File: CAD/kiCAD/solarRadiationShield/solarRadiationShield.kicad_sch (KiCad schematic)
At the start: 4 parts, among them J3 INSIG

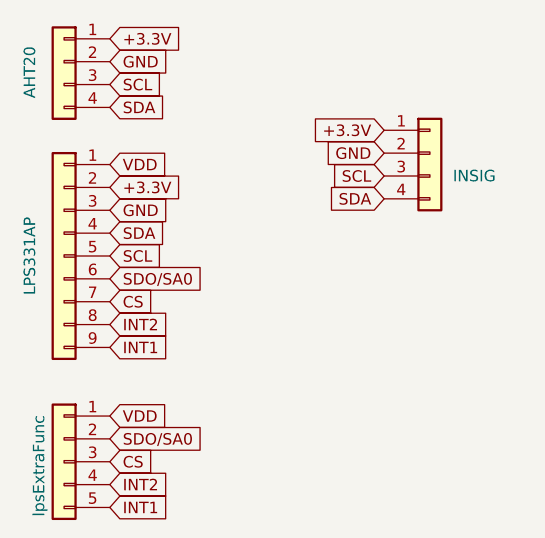
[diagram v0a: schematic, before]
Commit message: Big Updates
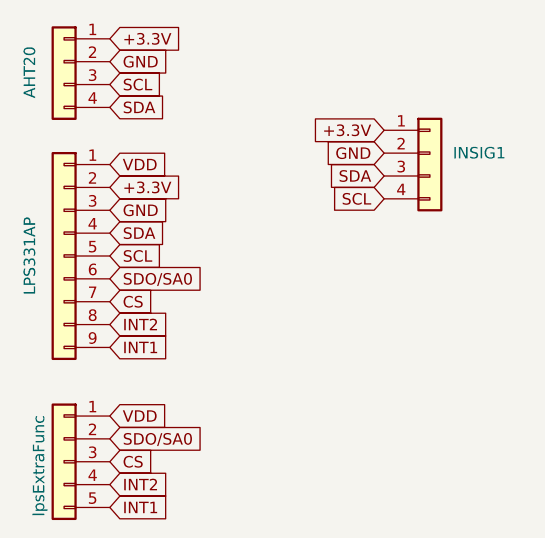
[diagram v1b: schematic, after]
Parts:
- renumbered J3 to INSIG1
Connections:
- net SCL: now also INSIG1.4 (Pin_4); no longer INSIG1.3 (Pin_3)
- net SDA: now also INSIG1.3 (Pin_3); no longer INSIG1.4 (Pin_4)
